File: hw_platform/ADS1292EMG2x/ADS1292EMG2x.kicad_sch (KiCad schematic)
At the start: 36 parts

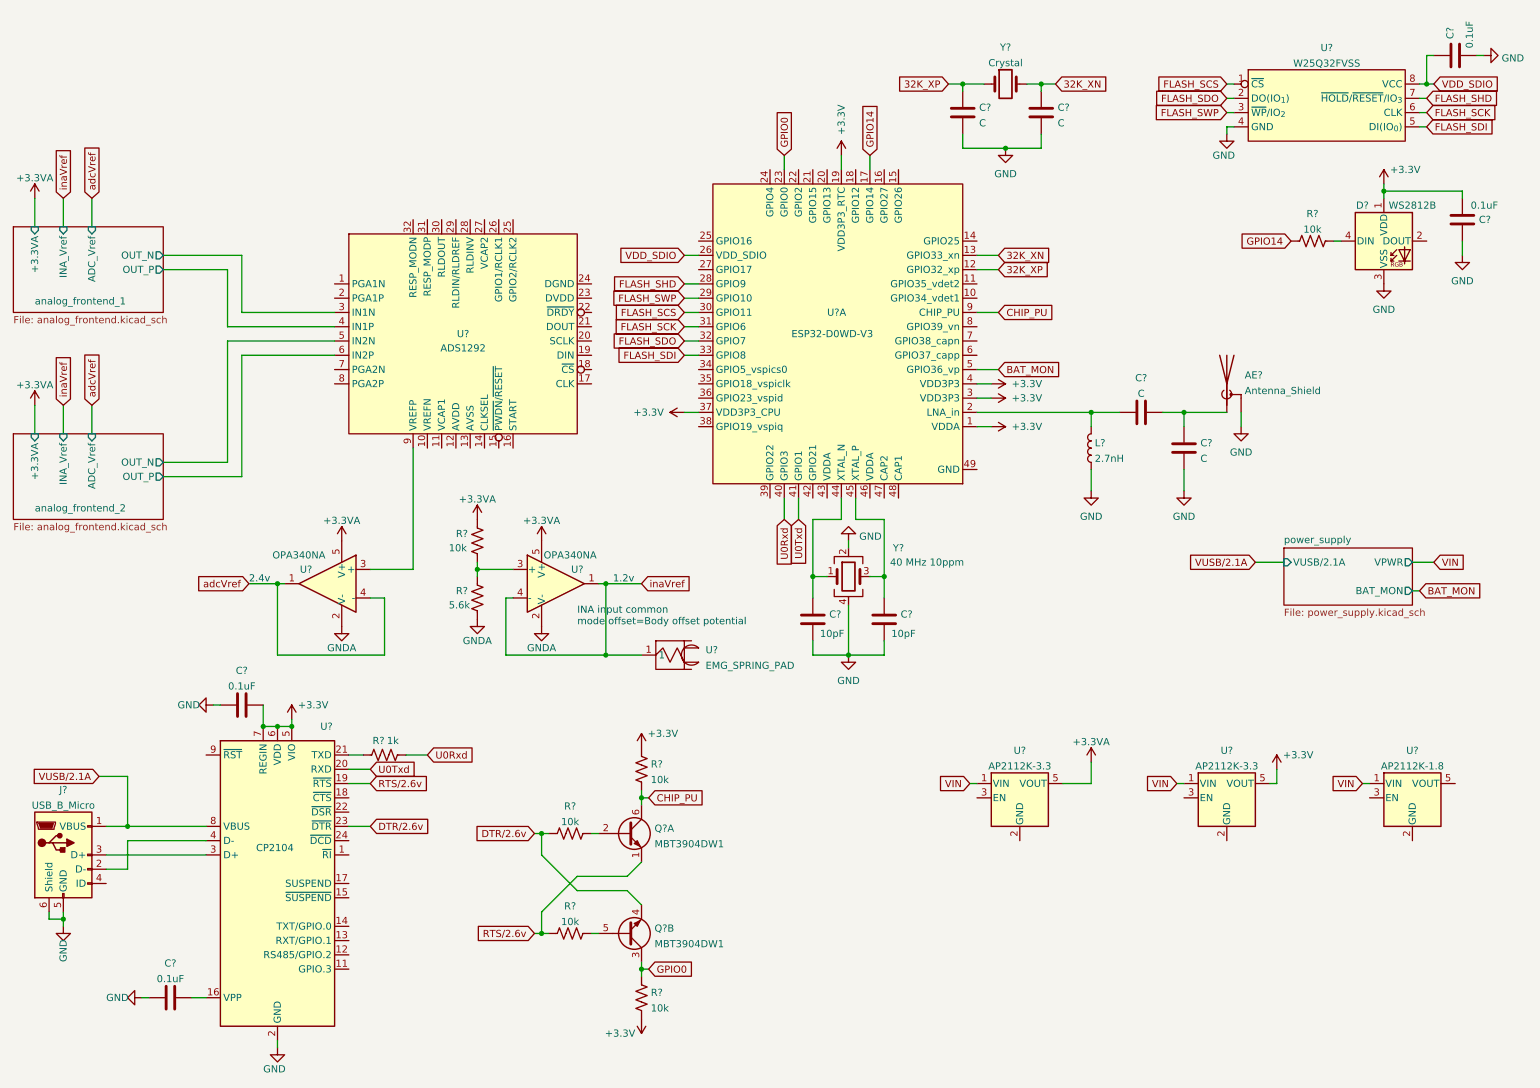
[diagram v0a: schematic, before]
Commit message: schematic verification
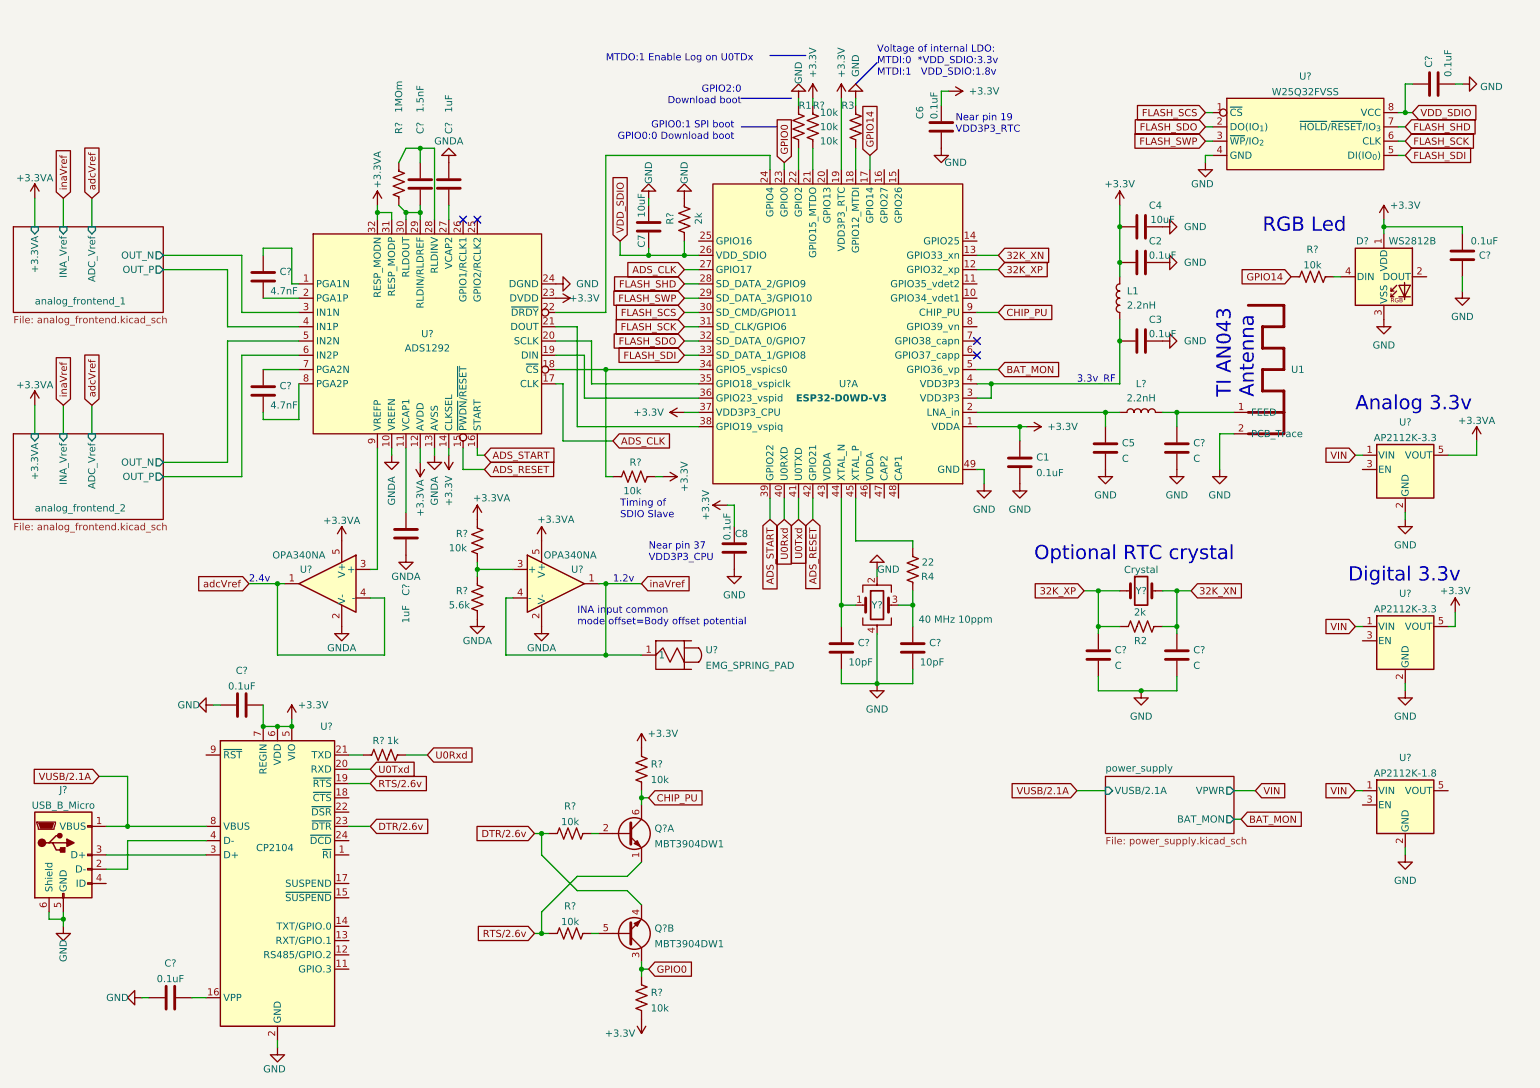
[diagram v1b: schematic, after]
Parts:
- removed AE?: Antenna_Shield, symbol Device:Antenna_Shield
- removed C?: C, symbol Device:C
- added C1, C2, C3, C6, C8: 0.1uF, symbol Device:C
- added C4, C7: 10uF, symbol Device:C
- added C5: C, symbol Device:C
- added C? (x2): 4.7nF, symbol Device:C
- added C? (x2): 1uF, symbol Device:C
- added C?: 1.5nF, symbol Device:C
- added L1: 2.2nH, symbol Device:L
- added R1, R3, R? (x2): 10k, symbol Device:R_US
- added R2, R?: 2k, symbol Device:R_US
- added R4: 22, symbol Device:R_US
- added R?: 1MOm, symbol Device:R_US
- added U1: ~, symbol espLib:PCB_Antenna_2.4GHz_50Jhm
- L?: value 2.7nH -> 2.2nH
- U? (x2): Spice_Lib_File libs\OPA340.LIB -> (none); Spice_Model OPA340 -> (none); Spice_Netlist_Enabled Y -> (none); Spice_Node_Sequence 3 4 5 2 1 -> (none); Spice_Primitive X -> (none)
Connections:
- net +3.3VA: now also U?.12 (AVDD), U?.31 (RESP_MODP), U?.32 (RESP_MODN)
- net 32K_XN: now also R2.2
- net 32K_XP: now also R2.1
- net GND: now also U?.2 (GND), U?.2 (GND), U?.2 (GND), U?.24 (DGND), U?.49 (GND), C1.2, C2.2, C3.2, C4.2, C5.1, C6.1, C7.2, C8.1, R1.2, R3.2, R?.1, U1.2 (PCB_Trace); no longer L?.1
- net GNDA: now also U?.10 (VREFN), U?.13 (AVSS), C?.1, C?.1
- net VDD_SDIO: now also C7.1, R?.2
- net at U?.18 (GPIO12_MTDI): now also R3.1
- net at L?.2: now also C?.2, U1.1 (FEED); no longer U?.2 (LNA_in)
- net at U?.21 (GPIO15_MTDO): now also R?.1
- net at U?.22 (GPIO2): now also R1.1
- net at U?.24 (GPIO4): now also U?.22 (~{DRDY})
- net ADS_CLK: now reaches U?.27 (GPIO17)
- net ADS_CLK: now also U?.17 (CLK)
- net at U?.34 (GPIO5_vspics0): now also U?.18 (~{CS}), R?.2
- net at U?.35 (GPIO18_vspiclk): now also U?.20 (SCLK)
- net at U?.36 (GPIO23_vspid): now also U?.19 (DIN)
- net at U?.38 (GPIO19_vspiq): now also U?.21 (DOUT)
- net ADS_START: now reaches U?.39 (GPIO22)
- net ADS_START: now also U?.16 (START)
- net ADS_RESET: now reaches U?.42 (GPIO21)
- net ADS_RESET: now also U?.15 (~{PWDN}/~{RESET})
- net at C?.1, Y?.3: now also R4.2; no longer U?.45 (XTAL_P)
- net at U?.1 (PGA1N): now also C?.1
- net at U?.11 (VCAP1): now also C?.2
- net +3.3V: now reaches U?.14 (CLKSEL)
- net +3.3V: now also C?.2, C?.2, D?.1 (VDD), R?.1, R?.2, U?.1 (VDDA), U?.19 (VDD3P3_RTC), U?.23 (DVDD), U?.37 (VDD3P3_CPU), U?.5 (VIO), U?.5 (VOUT), U?.6 (VDD), U?.7 (REGIN), C1.1, C2.1, C4.1, C6.2, C8.2, L1.2, R?.1, R?.2
- net at U?.2 (PGA1P): now also C?.2
- net at U?.27 (VCAP2): now also C?.2
- net at U?.28 (RLDINV): now also C?.1, R?.2
- net at U?.29 (RLDIN/RLDREF): now also U?.30 (RLDOUT), C?.2, R?.1
- net at U?.7 (PGA2N): now also C?.1
- net at U?.8 (PGA2P): now also C?.2
- removed net +3V3: C?.2, C?.2, D?.1 (VDD), R?.1, R?.2, U?.1 (VDDA), U?.19 (VDD3P3_RTC), U?.3 (VDD3P3), U?.37 (VDD3P3_CPU), U?.4 (VDD3P3), U?.5 (VIO), U?.5 (VOUT), U?.6 (VDD), U?.7 (REGIN)
- new net: C3.1, L1.1, U?.3 (VDD3P3), U?.4 (VDD3P3)
- new net: C5.2, L?.1, U?.2 (LNA_in)
- new net: R4.1, U?.45 (XTAL_P)
- no-connect marks 0 -> 4
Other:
- note added: "3.3v_RF"
- note added: "Analog 3.3v"
- note added: "Digital 3.3v"
- note added: "GPIO0:1 SPI boot GPIO0:0 Download boot"
- note added: "GPIO2:0 Download boot"
- note added: "MTDO:1 Enable Log on U0TDx"
- note added: "Near pin 19 VDD3P3_RTC"
- note added: "Near pin 37 VDD3P3_CPU"
- note added: "Optional RTC crystal"
- note added: "RGB Led"
- note added: "TI AN043 Antenna"
- note added: "Timing of SDIO Slave"
- note added: "Voltage of internal LDO: MTDI:0 *VDD_SDIO:3.3v MTDI:1 VDD_SDIO:1.8v"
- moved on the sheet: C?, D?, L?, R?, U?, Y?
